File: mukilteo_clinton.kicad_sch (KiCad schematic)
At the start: 22 parts

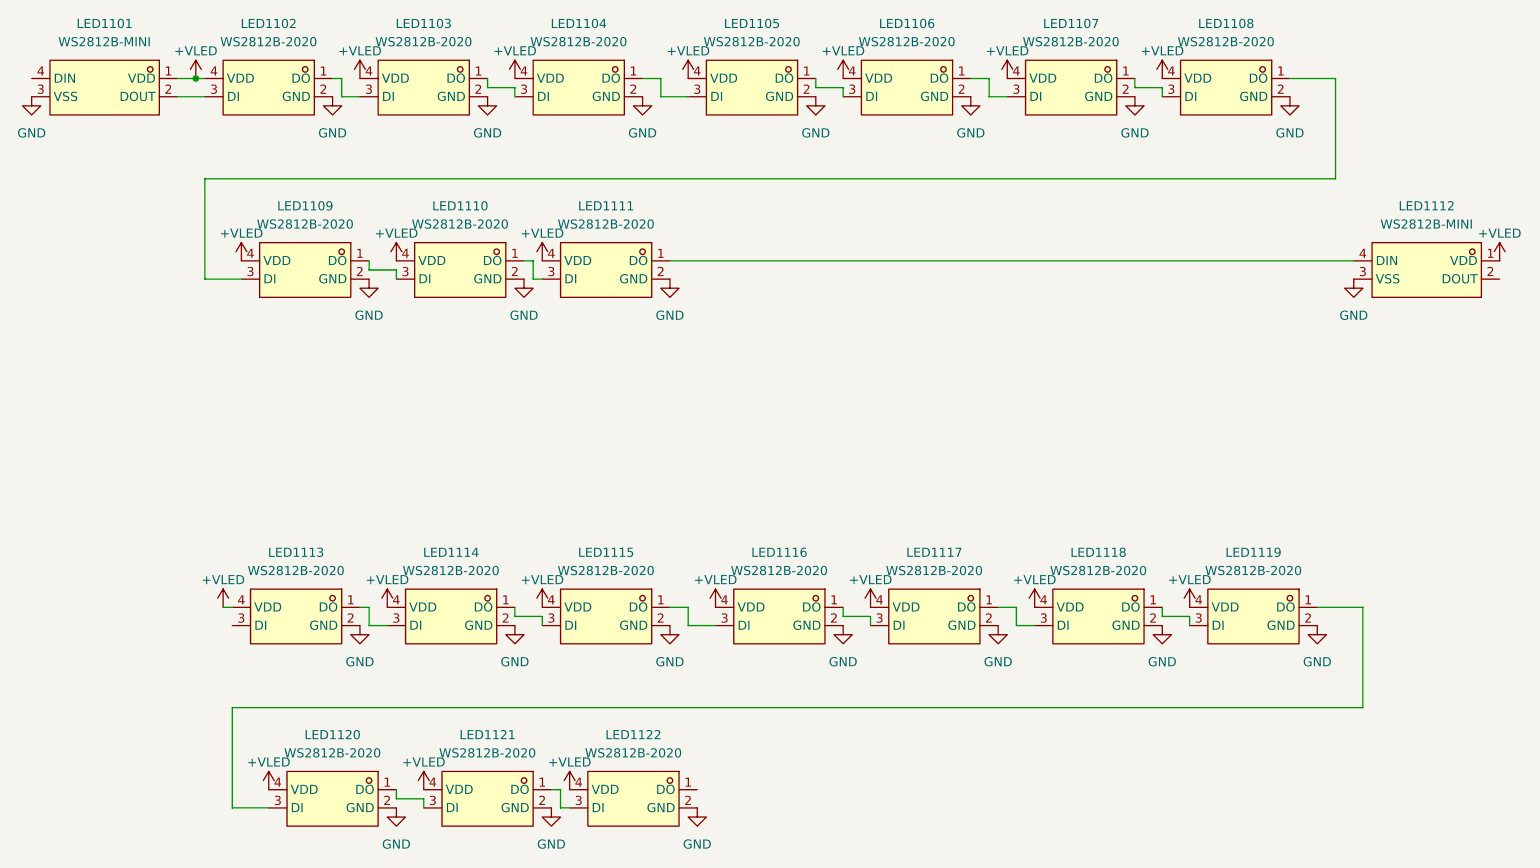
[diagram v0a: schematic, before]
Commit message: checkpoint before label plugin
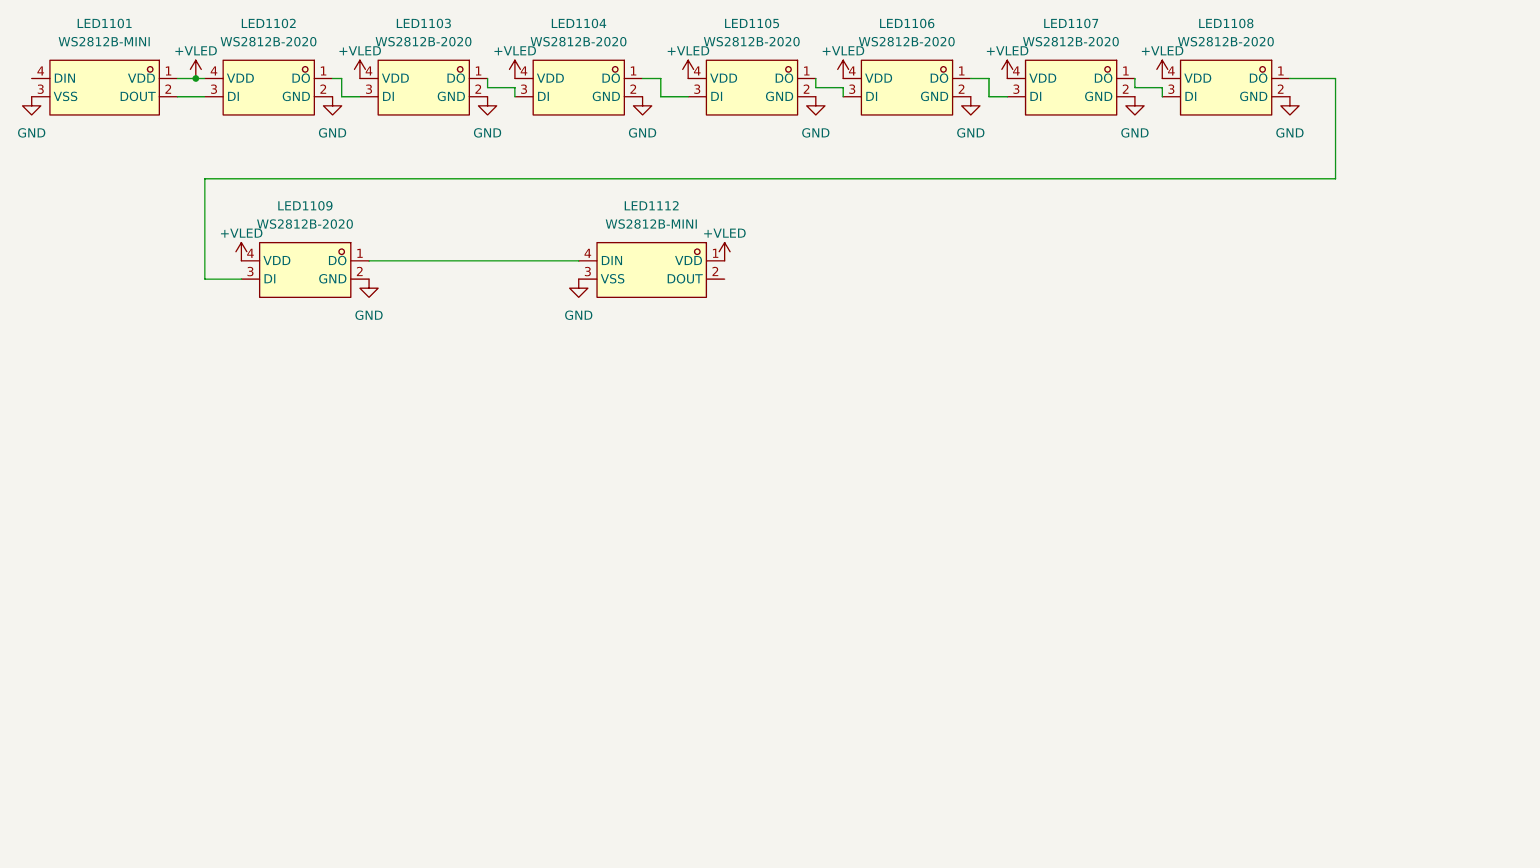
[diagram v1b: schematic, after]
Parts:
- removed LED1110, LED1111, LED1113, LED1114, LED1115, LED1116, LED1117, LED1118, LED1119, LED1120, LED1121, LED1122: WS2812B-2020, EasyEDA:LED-SMD_4P-L2.0-W2.0-TL_WS2812B-2020, symbol EasyEDA:WS2812B-2020
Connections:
- net at LED1109.1 (DO): now also LED1112.4 (DIN)
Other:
- moved on the sheet: LED1112
